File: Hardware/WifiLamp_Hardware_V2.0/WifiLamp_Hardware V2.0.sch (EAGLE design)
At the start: 24 parts, among them CN1 MKDSN1,5/2-5,08, CN3 MKDSN1,5/2-5,08, CN4 MKDSN1,5/2-5,08, T1 BTA12, U1 LM1117, U2 MOC3041M

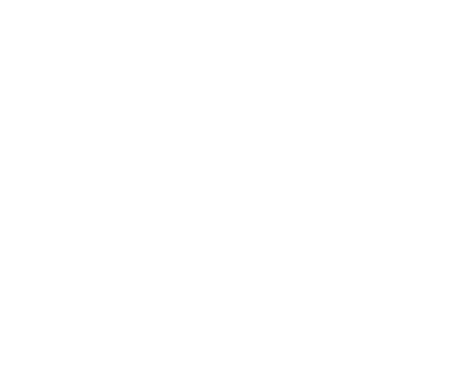
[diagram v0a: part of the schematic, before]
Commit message: Inclusao do firmware e app
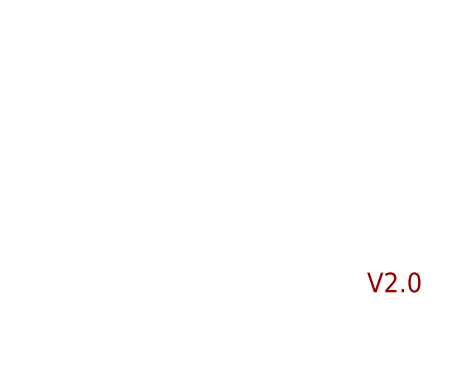
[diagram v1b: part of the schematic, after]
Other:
- note added: "V2.0"
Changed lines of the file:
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@@
 <?xml version="1.0" encoding="utf-8"?>
 <!DOCTYPE eagle SYSTEM "eagle.dtd">
-<eagle version="7.7.0">
+<eagle version="7.6.0">
 <drawing>
 <settings>
@@
 <grid distance="0.1" unitdist="inch" unit="inch" style="lines" multiple="1" display="no" altdistance="0.01" altunitdist="inch" altunit="inch"/>
 <layers>
-<layer number="1" name="Top" color="4" fill="1" visible="no" active="no"/>
-<layer number="16" name="Bottom" color="1" fill="1" visible="no" active="no"/>
-<layer number="17" name="Pads" color="2" fill="1" visible="no" active="no"/>
-<layer number="18" name="Vias" color="2" fill="1" visible="no" active="no"/>
-<layer number="19" name="Unrouted" color="6" fill="1" visible="no" active="no"/>
-<layer number="20" name="Dimension" color="15" fill="1" visible="no" active="no"/>
-<layer number="21" name="tPlace" color="7" fill="1" visible="no" active="no"/>
-<layer number="22" name="bPlace" color="7" fill="1" visible="no" active="no"/>
-<layer number="23" name="tOrigins" color="15" fill="1" visible="no" active="no"/>
-<layer number="24" name="bOrigins" color="15" fill="1" visible="no" active="no"/>
-<layer number="25" name="tNames" color="7" fill="1" visible="no" active="no"/>
-<layer number="26" name="bNames" color="7" fill="1" visible="no" active="no"/>
-<layer number="27" name="tValues" color="7" fill="1" visible="no" active="no"/>
-<layer number="28" name="bValues" color="7" fill="1" visible="no" active="no"/>
+<layer number="1" name="Top" color="4" fill="1" visible="yes" active="no"/>
+<layer number="16" name="Bottom" color="1" fill="1" visible="yes" active="no"/>
+<layer number="17" name="Pads" color="2" fill="1" visible="yes" active="no"/>
+<layer number="18" name="Vias" color="2" fill="1" visible="yes" active="no"/>
+<layer number="19" name="Unrouted" color="6" fill="1" visible="yes" active="no"/>
+<layer number="20" name="Dimension" color="15" fill="1" visible="yes" active="no"/>
+<layer number="21" name="tPlace" color="7" fill="1" visible="yes" active="no"/>
+<layer number="22" name="bPlace" color="7" fill="1" visible="yes" active="no"/>
+<layer number="23" name="tOrigins" color="15" fill="1" visible="yes" active="no"/>
+<layer number="24" name="bOrigins" color="15" fill="1" visible="yes" active="no"/>
+<layer number="25" name="tNames" color="7" fill="1" visible="yes" active="no"/>
+<layer number="26" name="bNames" color="7" fill="1" visible="yes" active="no"/>
+<layer number="27" name="tValues" color="7" fill="1" visible="yes" active="no"/>
+<layer number="28" name="bValues" color="7" fill="1" visible="yes" active="no"/>
 <layer number="29" name="tStop" color="7" fill="3" visible="no" active="no"/>
 <layer number="30" name="bStop" color="7" fill="6" visible="no" active="no"/>
@@
 <layer number="35" name="tGlue" color="7" fill="4" visible="no" active="no"/>
 <layer number="36" name="bGlue" color="7" fill="5" visible="no" active="no"/>
-<layer number="37" name="tTest" color="7" fill="1" visible="no" active="no"/>
-<layer number="38" name="bTest" color="7" fill="1" visible="no" active="no"/>
+<layer number="37" name="tTest" color="7" fill="1" visible="yes" active="no"/>
+<layer number="38" name="bTest" color="7" fill="1" visible="yes" active="no"/>
 <layer number="39" name="tKeepout" color="4" fill="11" visible="no" active="no"/>
 <layer number="40" name="bKeepout" color="1" fill="11" visible="no" active="no"/>
@@
 <layer number="44" name="Drills" color="7" fill="1" visible="no" active="no"/>
 <layer number="45" name="Holes" color="7" fill="1" visible="no" active="no"/>
-<layer number="46" name="Milling" color="3" fill="1" visible="no" active="no"/>
-<layer number="47" name="Measures" color="7" fill="1" visible="no" active="no"/>
-<layer number="48" name="Document" color="7" fill="1" visible="no" active="no"/>
-<layer number="49" name="Reference" color="7" fill="1" visible="no" active="no"/>
-<layer number="51" name="tDocu" color="7" fill="1" visible="no" active="no"/>
-<layer number="52" name="bDocu" color="7" fill="1" visible="no" active="no"/>
+<layer number="46" name="Milling" color="3" fill="1" visible="yes" active="no"/>
+<layer number="47" name="Measures" color="7" fill="1" visible="yes" active="no"/>
+<layer number="48" name="Document" color="7" fill="1" visible="yes" active="no"/>
+<layer number="49" name="Reference" color="7" fill="1" visible="yes" active="no"/>
+<layer number="51" name="tDocu" color="7" fill="1" visible="yes" active="no"/>
+<layer number="52" name="bDocu" color="7" fill="1" visible="yes" active="no"/>
 <layer number="90" name="Modules" color="5" fill="1" visible="yes" active="yes"/>
 <layer number="91" name="Nets" color="2" fill="1" visible="yes" active="yes"/>
@@
 Embarcados
 Mazza-G Tec</text>
+<text x="250.19" y="15.24" size="2.1844" layer="94">V2.0</text>
 </plain>
 <instances>
